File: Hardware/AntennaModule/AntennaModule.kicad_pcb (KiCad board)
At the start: 2 copper layers, 80 x 80 mm, 53 parts, among them J1 Conn_01x10, SW1 ColdStart, U1 C0727J5003AHF-1, U2 C0727J5003AHF-1, U3 NJG1155UX2, U4 NT1192FAAE1S, U5 PD0922J5050S2HF, U6 NT1192FAAE1S, U7 NEO-D9C, U8 NEO-F9P, X1 TA1985A, X2 TE0133B

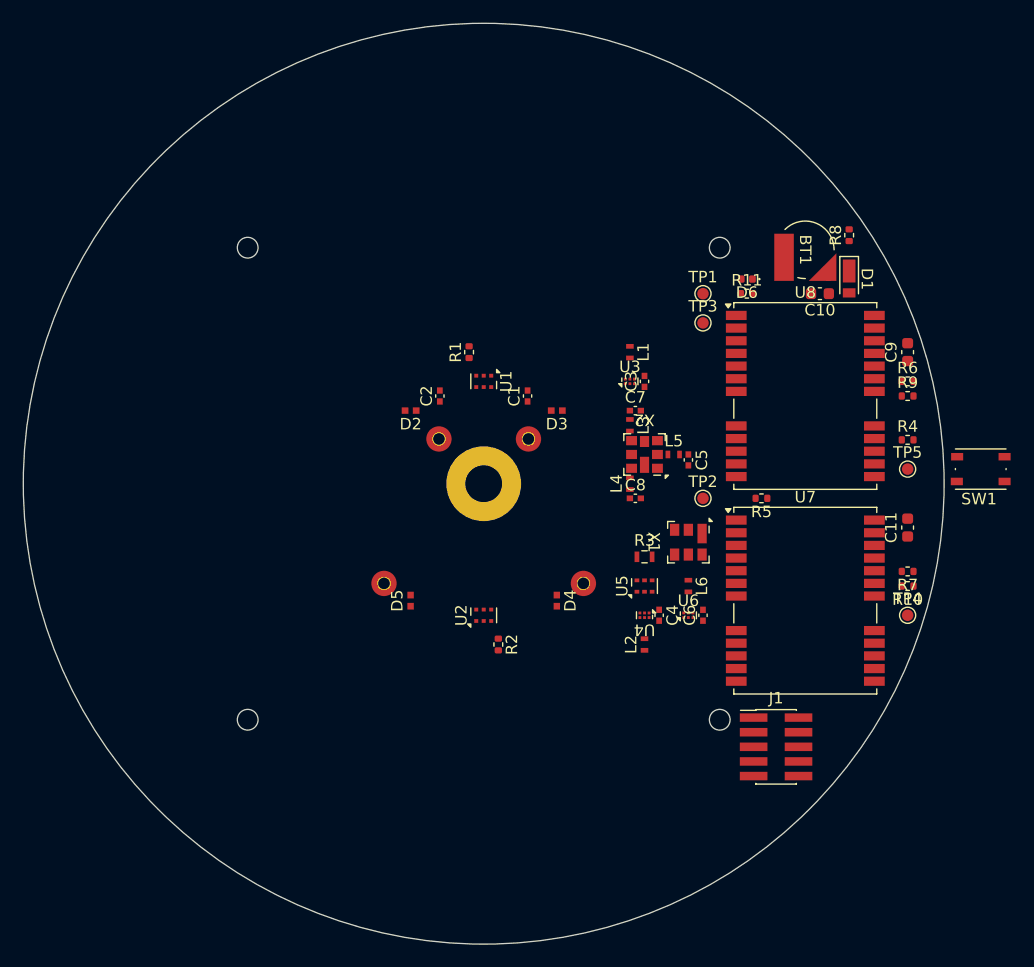
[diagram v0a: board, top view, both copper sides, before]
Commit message: スタックアップを決定
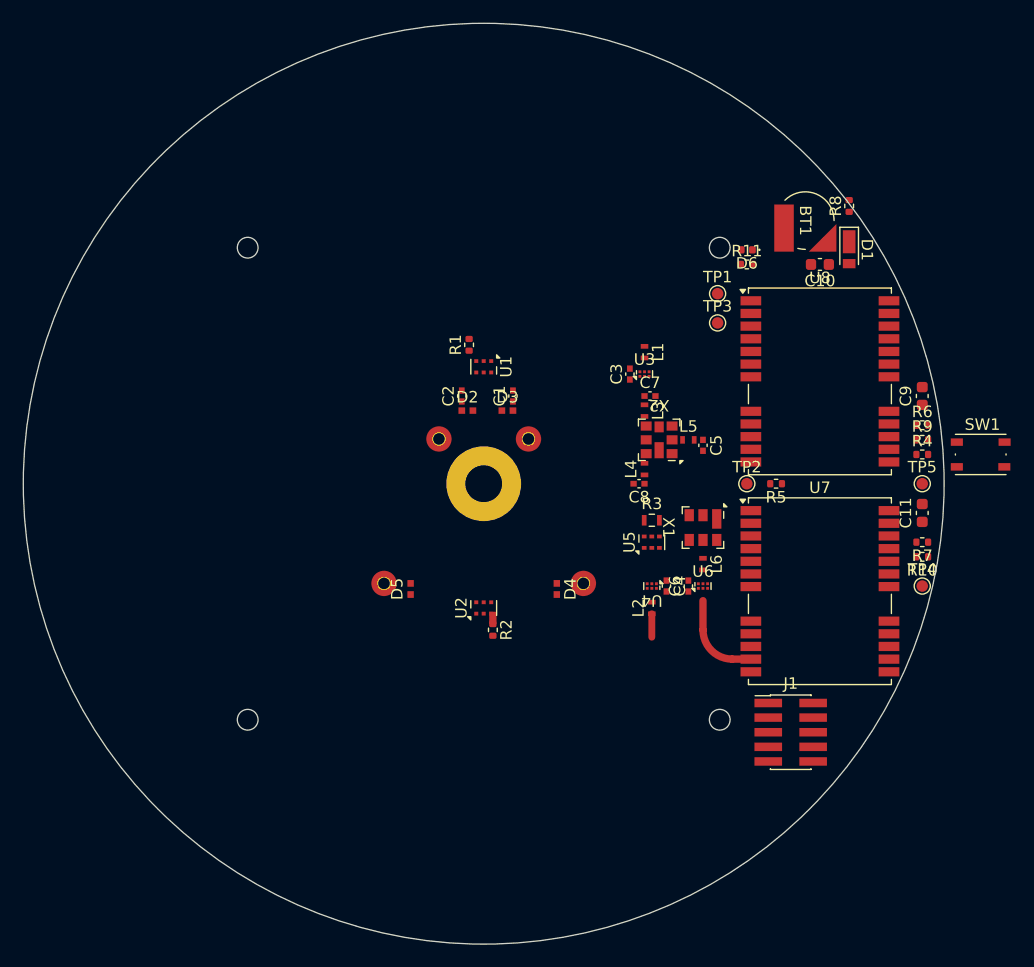
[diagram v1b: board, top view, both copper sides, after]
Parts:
- moved D2 4.93 mm to (148.6, 93.7), turned to 0 degrees
- moved D3 4.29 mm to (152.1, 93.7), turned to 0 degrees
- moved TP2 4.02 mm to (172.9, 100.0)
- moved C9 4.02 mm to (188.1, 92.4)
- moved R6 4.02 mm to (188.1, 94.9)
- moved R9 4.02 mm to (188.1, 96.2)
- moved U5 3.86 mm to (164.6, 105.1)
- moved L2 3.24 mm to (164.6, 110.8)
- moved R3 3.24 mm to (164.6, 103.2)
- moved C6 2.84 mm to (167.8, 108.9)
- moved U6 2.84 mm to (169.1, 108.9)
- moved R10 2.84 mm to (188.1, 106.3)
- moved R7 2.84 mm to (188.1, 105.1)
- moved TP4 2.84 mm to (188.1, 108.9)
- moved C4 2.62 mm to (165.9, 108.9)
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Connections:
- C3 pad 1: +3.3VA -> +3.3VP
- U3 pad 2: +3.3VA -> +3.3VP
- U3 pad 6: +3.3VA -> +3.3VP
- U7 pad 9: unconnected-(U7-VCC_RF-Pad9) -> +3.3VA
- U8 pad 9: +3.3VA -> +3.3VP
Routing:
- net /RF_IN_D9C: track 0.00 -> 8.05 mm
- net Net-(U2-Input): track 0.00 -> 2.03 mm
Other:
- copper layers 2 -> 4
- board text added: "0"
- board text added: "0 mm"
- board text added: "0.01 mm"
- board text added: "0.0152 mm"
- board text added: "0.02"
- board text added: "0.035 mm"
- board text added: "0.1000 mm / 0.1000 mm"
- board text added: "0.1164 mm"
- board text added: "0.1500 mm"
- board text added: "0.218 mm"
- board text added: "0.4 mm"
- board text added: "0.4mm H/HOZ without copper"
- board text added: "1"
- board text added: "1.6252 mm"
- board text added: "2116 RC54% 4.9mil"
- board text added: "3.8"
- board text added: "4"
- board text added: "4.4"
- board text added: "4.6"
- board text added: "7628, RC 49%, 8.6 mil"
- board text added: "80.0025 mm x 80.0025 mm"
- board text added: "B.Cu"
- board text added: "B.Mask"
- board text added: "B.Paste"
- board text added: "B.Silkscreen"
- board text added: "Bottom Silk Screen"
- board text added: "Bottom Solder Mask"
- board text added: "Bottom Solder Paste"
- board text added: "ENIG"
- board text added: "F.Cu"
- board text added: "F.Mask"
- board text added: "F.Paste"
- board text added: "F.Silkscreen"
- board text added: "In1.Cu"
- board text added: "In2.Cu"
- board text added: "JLC04161H-7628B"
- board text added: "Not specified"
- board text added: "RFINパッドの高さを揃える"
- board text added: "Top Silk Screen"
- board text added: "Top Solder Mask"
- board text added: "Top Solder Paste"
- board text added: "copper"
- board text added: "core"
- board text added: "prepreg"
- board text added: "εR"
- board text added: "いいえ"
- board text added: "はい"
- board text added: "インピーダンス制御:"
- board text added: "エッジ カード コネクタ:"
- board text added: "カラー"
- board text added: "タイプ"
- board text added: "レイヤー名"
- board text added: "基板の特性"
- board text added: "基板全体の寸法:"
- board text added: "基板厚:"
- board text added: "基板端メッキ:"
- board text added: "導体レイヤー数:"
- board text added: "損失正接"
- board text added: "曲げ半径は配線幅の3倍以上 抵抗の中心xは接続するパッドの中心xから外側に0.145オフセット 下側TVSダイオード位置合わせ済"
- board text added: "最小穴径:"
- board text added: "最小配線幅/間隔:"
- board text added: "材料"
- board text added: "端面スルーホール パッド:"
- board text added: "線幅 (mm)"
- board text added: "誘電体 1 (1/3)"
- board text added: "誘電体 2"
- board text added: "誘電体 3 (1/3)"
- board text added: "銅箔仕上げ:"
